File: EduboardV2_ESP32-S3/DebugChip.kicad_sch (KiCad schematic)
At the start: 31 parts, among them Q1 L8050QLT1G, Q2 L8050QLT1G, Q3 AO3401A, U2 CP2102N-A02-GQFN28R

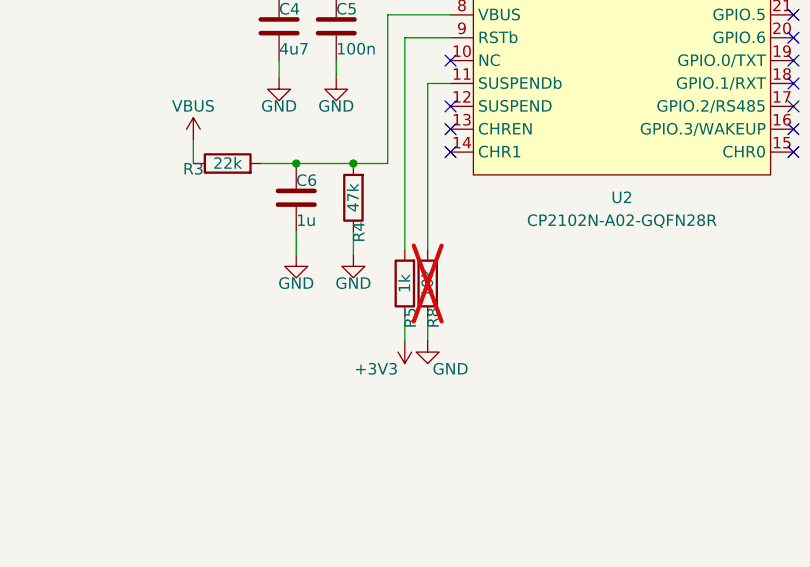
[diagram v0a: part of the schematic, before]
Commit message: finish schematic. Do Layout
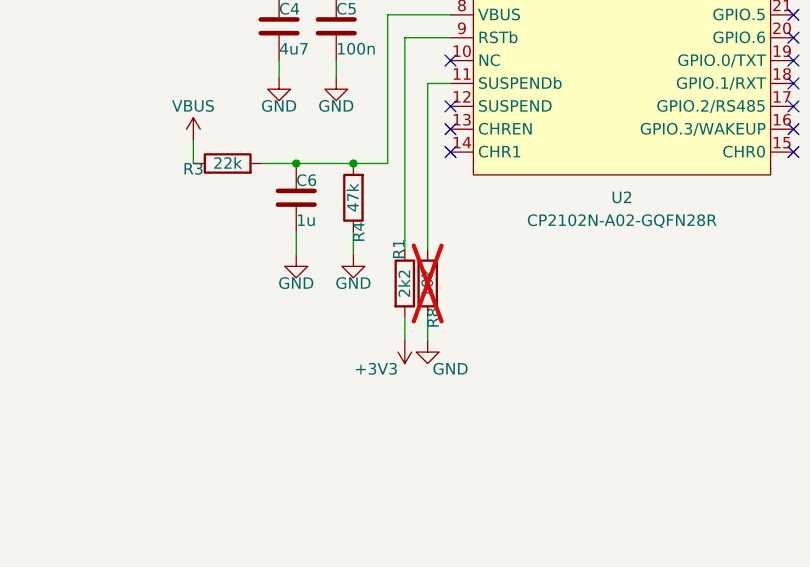
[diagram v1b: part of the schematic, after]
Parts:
- removed R5: 1k, Resistor_SMD:R_0603_1608Metric, symbol Device:R
- added R1: 2k2, Resistor_SMD:R_0402_1005Metric, symbol Device:R
- C6: JLCPCB Part # (none) -> C77083; LCSC Part (none) -> C77083
- Q1, Q2: JLCPCB Part # (none) -> C49581
- R10, R13, R14, R9: footprint Resistor_SMD:R_0603_1608Metric -> Resistor_SMD:R_0402_1005Metric; JLCPCB Part # (none) -> C140225; LCSC Part (none) -> C140225
- R11, R12, R8: footprint Resistor_SMD:R_0603_1608Metric -> Resistor_SMD:R_0402_1005Metric; JLCPCB Part # (none) -> C71617; LCSC Part (none) -> C71617
- R25: footprint Resistor_SMD:R_0603_1608Metric -> Resistor_SMD:R_0402_1005Metric; JLCPCB Part # C115003 -> C114762; LCSC Part C115003 -> C114762
- R3: footprint Resistor_SMD:R_0603_1608Metric -> Resistor_SMD:R_0402_1005Metric; JLCPCB Part # (none) -> C144778; LCSC Part (none) -> C144778
- R31, R32: footprint Resistor_SMD:R_0603_1608Metric -> Resistor_SMD:R_0402_1005Metric; JLCPCB Part # C465460 -> C140225; LCSC Part C465460 -> C140225
- R4: footprint Resistor_SMD:R_0603_1608Metric -> Resistor_SMD:R_0402_1005Metric; JLCPCB Part # (none) -> C328320; LCSC Part (none) -> C328320
- R6, R7: footprint Resistor_SMD:R_0603_1608Metric -> Resistor_SMD:R_0402_1005Metric; JLCPCB Part # C116677 -> C71617; LCSC Part C116677 -> C71617
- U2: footprint easyeda2kicad:QFN-28_L5.0-W5.0-P0.50-TL-EP3.3 -> EduboardV2_kicadlib:QFN-28_L5.0-W5.0-P0.50-TL-EP3.3; JLCPCB Part # (none) -> C964632
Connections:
- net +3V3: now also R1.2
- net at U2.9 (RSTb): now also R1.1
